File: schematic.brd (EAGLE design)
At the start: 100 x 59.7 mm, 25 parts

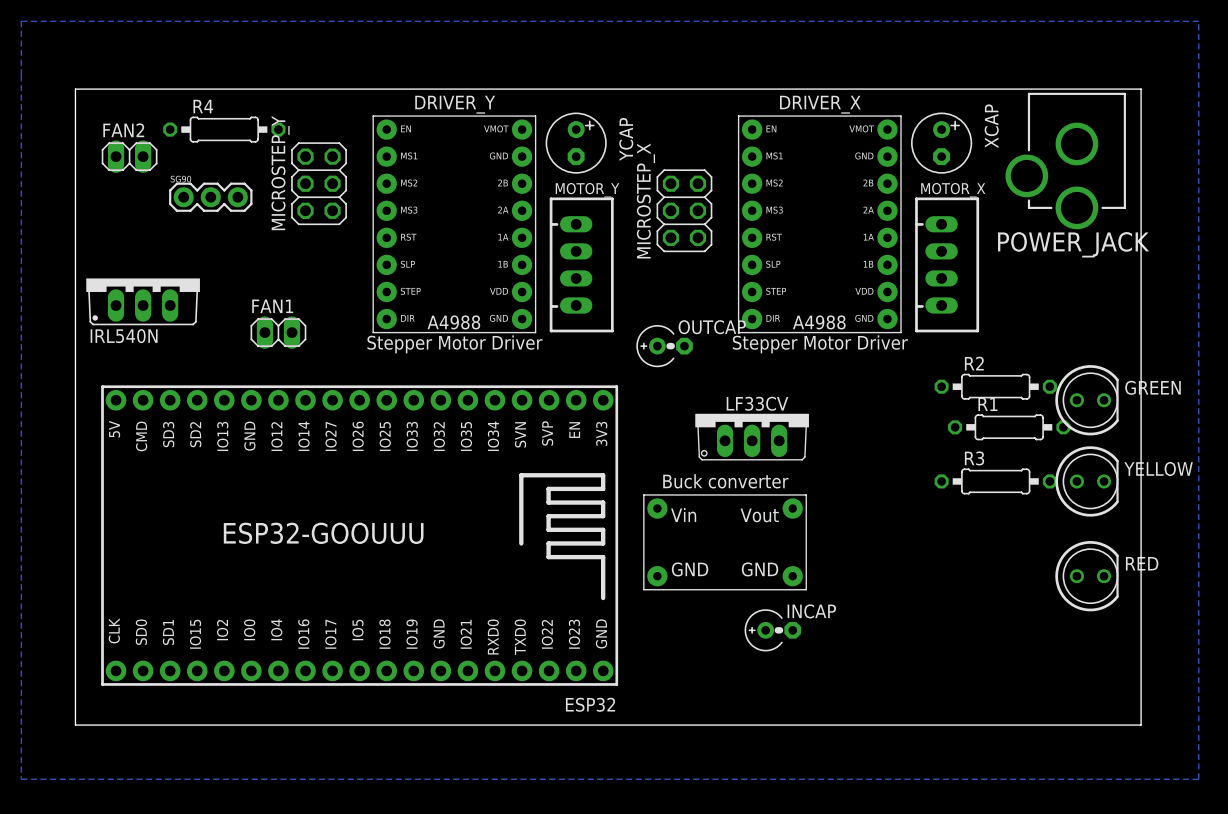
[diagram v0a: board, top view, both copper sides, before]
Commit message: akjdf;sjf
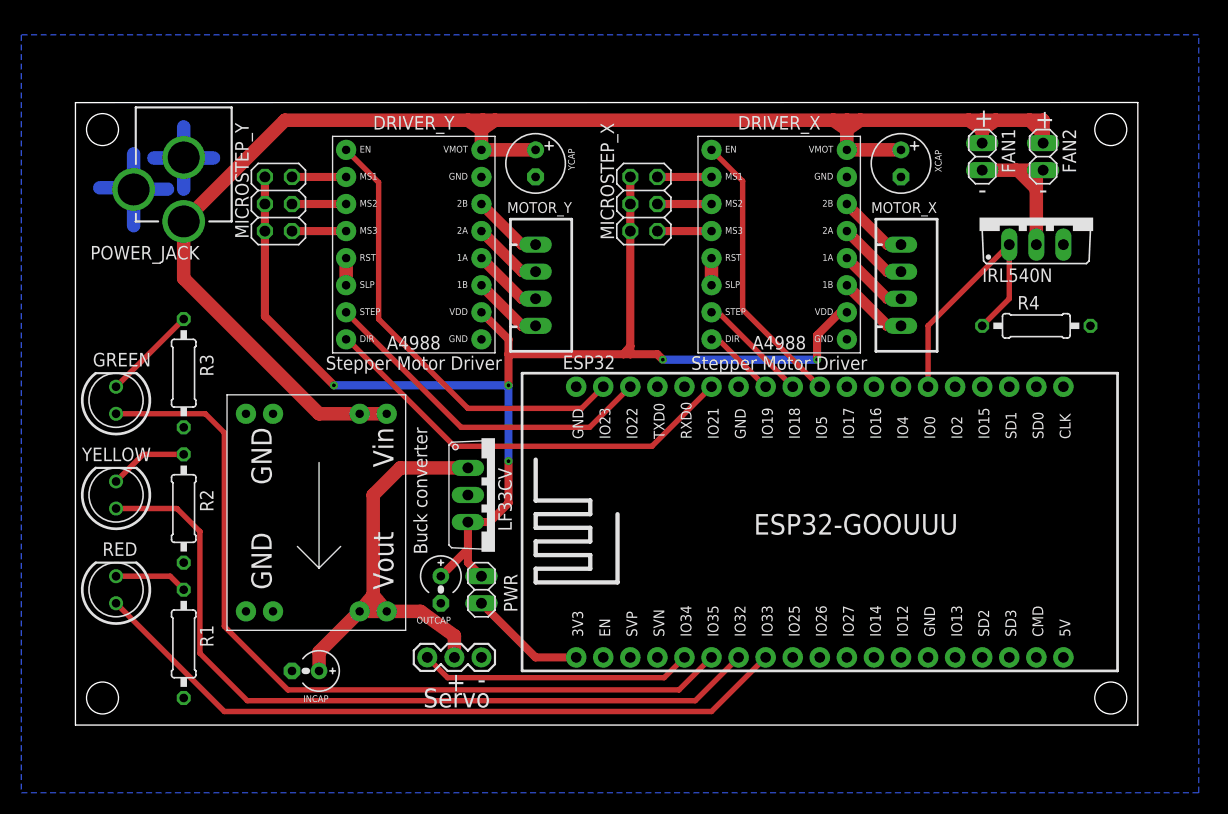
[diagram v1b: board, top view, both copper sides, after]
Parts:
- removed U$1: BUCK-CONVERTER, buck-converter:BUCK-CONVERTER
- added PWR: (no value), pinhead:1X02
- added U$2: BUCK-CONVERTER, mine:BUCK-CONVERTER
- moved RED 91.4 mm to (3.81, 12.7), turned to 90 degrees
- moved YELLOW 91.4 mm to (3.81, 21.6), turned to 90 degrees
- moved GREEN 91.4 mm to (3.81, 30.5), turned to 90 degrees
- moved FAN2 85.7 mm to (90.8, 53.3), turned to 270 degrees
- moved IRL540N 84.0 mm to (90.2, 47.6)
- moved POWER_JACK 83.8 mm to (10.2, 61.0)
- moved R1 80.1 mm to (10.2, 7.62), turned to 270 degrees
- moved R4 78.4 mm to (90.2, 37.5)
- moved R2 77.1 mm to (10.2, 20.3), turned to 270 degrees
- moved R3 76.9 mm to (10.2, 33.0), turned to 270 degrees
- moved FAN1 68.1 mm to (85.1, 53.3), turned to 270 degrees
- moved SG90 48.9 mm to (33.0, 6.35)
- moved INCAP 44.6 mm to (21.6, 5.08), turned to 180 degrees
- moved ESP32 43.2 mm to (69.8, 17.8), turned to 0 degrees
- moved OUTCAP 31.4 mm to (34.3, 12.7), turned to 270 degrees
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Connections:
- net MS1_X renamed N$11
- net MS1_Y renamed N$5
- net MS2_X renamed N$12
- net MS2_Y renamed N$9
- net MS3_X renamed N$13
- net MS3_Y renamed N$10
- net N$32 renamed FAN_PW
- removed net N$15: DRIVER_X./EN, ESP32.11
- removed net N$19: DRIVER_Y./EN, ESP32.8
- removed net N$2: DRIVER_X.STEP, ESP32.12
- removed net N$23: ESP32.37, RED.A
- removed net N$25: GREEN.K, R1.1
- removed net N$26: ESP32.33, GREEN.A
- removed net N$27: ESP32.36, YELLOW.A
- removed net N$29: R3.1, RED.K
- removed net N$30: ESP32.7, SG90.1
- removed net N$31: ESP32.28, IRL540N.G, R4.1
- removed net N$4: DRIVER_Y.DIR, ESP32.10
- removed net N$5 (its old number): DRIVER_Y.STEP, ESP32.9
- new net FAN_EN: ESP32.25, IRL540N.G, R4.1
- new net GREEN_LED: ESP32.6, GREEN.A
- new net N$21: R1.1, RED.K
- new net N$8: GREEN.K, R3.1
- new net RED_LED: ESP32.8, RED.A
- new net SERVO: ESP32.5, SG90.1
- new net X_DIR: DRIVER_X.DIR, ESP32.31
- new net X_EN: DRIVER_X./EN, ESP32.29
- new net X_STEP: DRIVER_X.STEP, ESP32.30
- new net YELLOW_LED: ESP32.7, YELLOW.A
- new net Y_DIR: DRIVER_Y.DIR, ESP32.33
- new net Y_EN: DRIVER_Y./EN, ESP32.37
- new net Y_STEP: DRIVER_Y.STEP, ESP32.36
- net +12V: now also U$2.VIN1, U$2.VIN2; no longer U$1.VIN
- net +3V3: now also PWR.2; no longer ESP32.1
- net +5V: now also U$2.VOUT1, U$2.VOUT2; no longer U$1.VOUT
- net GND: now also U$2.GND@1, U$2.GND@2, U$2.GND@3, U$2.GND@4; no longer U$1.GND@1, U$1.GND@2
- net N$1: now also ESP32.1, PWR.1; no longer DRIVER_X.DIR, ESP32.13
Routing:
- net +12V: track 0.00 -> 146.3 mm
- net +3V3: track 0.00 -> 124.1 mm, vias 0 -> 5
- net GREEN_LED: track 0.00 -> 78.5 mm
- net YELLOW_LED: track 0.00 -> 74.3 mm
- net RED_LED: track 0.00 -> 67.3 mm
- net Y_EN: track 0.00 -> 42.5 mm
- net +5V: track 0.00 -> 42.1 mm
- net Y_DIR: track 0.00 -> 40.8 mm
- net Y_STEP: track 0.00 -> 32.7 mm
- net X_EN: track 0.00 -> 26.4 mm
- net SERVO: track 0.00 -> 25.7 mm
- net FAN_EN: track 0.00 -> 25.2 mm
- net GND: track 0.00 -> 24.7 mm
- net FAN_PW: track 0.00 -> 15.4 mm
- net N$1: track 0.00 -> 11.0 mm
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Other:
- board size 100 x 59.7 mm -> 99.7 x 58.4 mm
- board text added: "+"
- board text added: "-"
- board text added: "Servo"
